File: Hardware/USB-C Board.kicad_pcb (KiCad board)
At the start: 2 copper layers, 34 x 34 mm, 52 parts, among them J1 USB_C_Receptacle_USB2.0, J2 Conn_01x04_Male, J3 Conn_01x02_Male, J4 Conn_01x02_Male, J5 Conn_01x02_Male, J6 Conn_01x02_Male, J9 Conn_01x04_MountingPin, Q1 DMP3013SFV, SW1 SW_Push, U1 AMS1117-3.3, U3 STUSB4500QTR

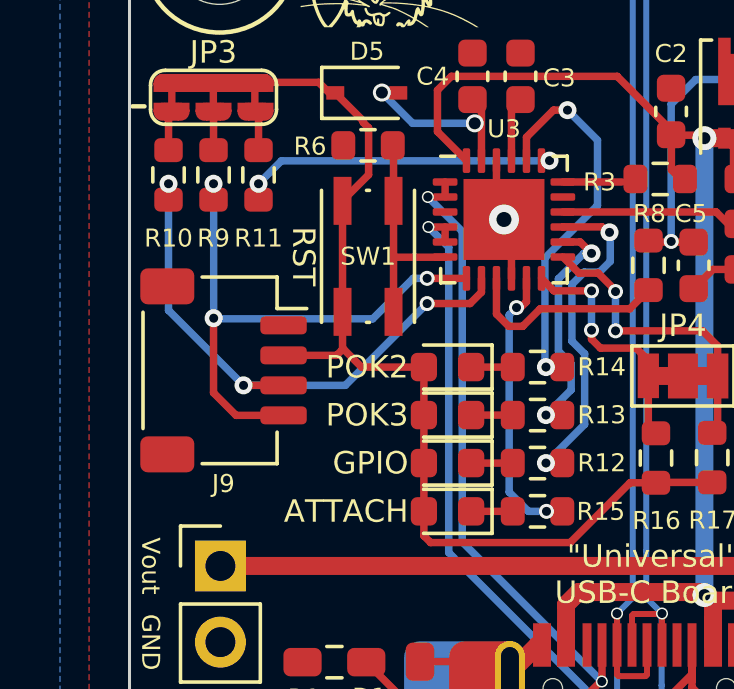
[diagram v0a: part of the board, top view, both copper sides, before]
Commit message: starting on controller boards
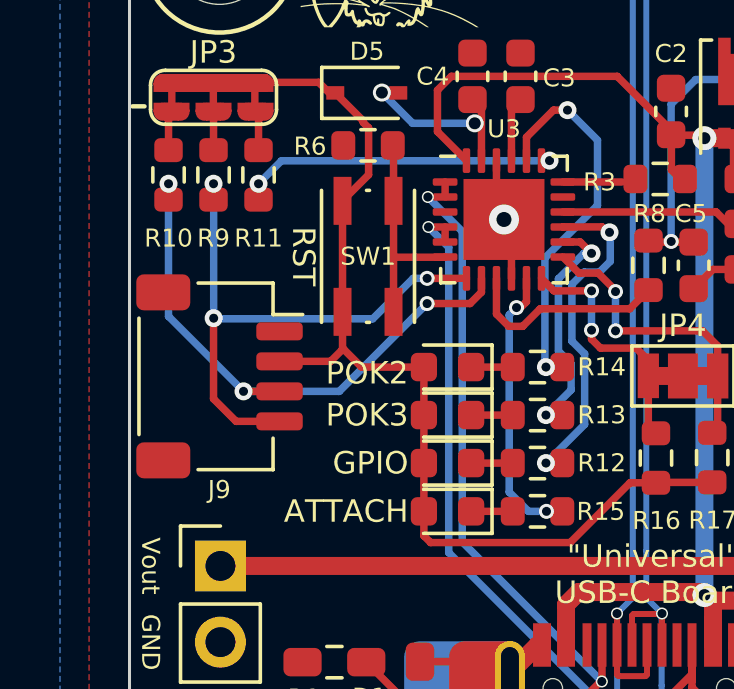
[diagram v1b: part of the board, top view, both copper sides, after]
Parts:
- moved J9 0.24 mm to (86.0, 87.0)
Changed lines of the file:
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@@
   )
   (footprint "Tinker:JST_SH_SM04B-SRSS-TB_1x04-1MP_P1.00mm_Horizontal" (layer "F.Cu")
-    (at 86.13441 86.8 -90)
+    (at 86 87 -90)
     (descr "JST SH series connector, SM04B-SRSS-TB (http://www.jst-mfg.com/product/pdf/eng/eSH.pdf), generated with kicad-footprint-generator")
     (tags "connector JST SH top entry")
@@
       (effects (font (size 0.6 0.6) (thickness 0.15)))
     )
-    (fp_text value "Conn_01x04_MountingPin" (at 0 3.98 -90) (layer "F.Fab") hide
+    (fp_text value "Conn_01x04_MountingPin" (at 0 3.98 90) (layer "F.Fab") hide
       (effects (font (size 1 1) (thickness 0.15)))
     )
-    (fp_text user "${REFERENCE}" (at 0 0 -90) (layer "F.Fab") hide
+    (fp_text user "${REFERENCE}" (at 0 0 90) (layer "F.Fab") hide
       (effects (font (size 1 1) (thickness 0.15)))
     )
@@
     (effects (font (size 0.6 0.6) (thickness 0.125)))
   )
-  (gr_text "POK2" (at 92.298126 86.690928) (layer "F.SilkS")
+  (gr_text "POK2" (at 92.298126 86.890928) (layer "F.SilkS")
     (effects (font (size 0.75 0.75) (thickness 0.15)) (justify right))
   )
@@
   (segment (start 99.675221 84.748251) (end 100.29898 84.124492) (width 0.25) (layer "F.Cu") (net 16))
   (segment (start 96.105782 85.332753) (end 96.690284 84.748251) (width 0.25) (layer "F.Cu") (net 16))
-  (segment (start 85.8 87.548526) (end 85.8 85.067178) (width 0.25) (layer "F.Cu") (net 17))
-  (segment (start 86.551474 88.3) (end 88.13441 88.3) (width 0.25) (layer "F.Cu") (net 17))
+  (segment (start 85.8 87.748526) (end 85.8 85.267178) (width 0.25) (layer "F.Cu") (net 17))
+  (segment (start 86.551474 88.5) (end 88.13441 88.5) (width 0.25) (layer "F.Cu") (net 17))
   (segment (start 85.8 85.067178) (end 85.805394 85.061784) (width 0.25) (layer "F.Cu") (net 17))
-  (segment (start 85.8 87.548526) (end 86.551474 88.3) (width 0.25) (layer "F.Cu") (net 17))
+  (segment (start 85.8 87.748526) (end 86.551474 88.5) (width 0.25) (layer "F.Cu") (net 17))
   (segment (start 94.231969 83.73369) (end 92.819469 83.73369) (width 0.25) (layer "F.Cu") (net 17))
   (via (at 92.919469 83.73369) (size 0.5) (drill 0.3) (layers "F.Cu" "B.Cu") (net 17))
@@
   (segment (start 85.805394 80.585394) (end 85.8 80.58) (width 0.25) (layer "B.Cu") (net 17))
   (segment (start 94.731969 83.73369) (end 94.731969 84.194198) (width 0.25) (layer "F.Cu") (net 18))
-  (segment (start 86.8 87.3) (end 88.13441 87.3) (width 0.25) (layer "F.Cu") (net 18))
+  (segment (start 86.8 87.5) (end 88.13441 87.5) (width 0.25) (layer "F.Cu") (net 18))
   (segment (start 94.731969 84.194198) (end 94.352345 84.573822) (width 0.25) (layer "F.Cu") (net 18))
   (segment (start 94.352345 84.573822) (end 92.819469 84.573822) (width 0.25) (layer "F.Cu") (net 18))
   (via (at 84.3 80.58) (size 0.6) (drill 0.3) (layers "F.Cu" "B.Cu") (net 18))
   (via (at 92.919469 84.573822) (size 0.5) (drill 0.3) (layers "F.Cu" "B.Cu") (net 18))
-  (via (at 86.8 87.3) (size 0.6) (drill 0.3) (layers "F.Cu" "B.Cu") (net 18))
-  (segment (start 90.193291 87.3) (end 92.919469 84.573822) (width 0.25) (layer "B.Cu") (net 18))
-  (segment (start 84.3 84.8) (end 84.3 80.58) (width 0.25) (layer "B.Cu") (net 18))
-  (segment (start 86.8 87.3) (end 90.193291 87.3) (width 0.25) (layer "B.Cu") (net 18))
-  (segment (start 86.8 87.3) (end 84.3 84.8) (width 0.25) (layer "B.Cu") (net 18))
+  (via (at 86.8 87.5) (size 0.6) (drill 0.3) (layers "F.Cu" "B.Cu") (net 18))
+  (segment (start 86.801247 87.501247) (end 89.992045 87.501247) (width 0.25) (layer "B.Cu") (net 18))
+  (segment (start 84.3 85) (end 84.3 80.58) (width 0.25) (layer "B.Cu") (net 18))
+  (segment (start 86.8 87.5) (end 86.801247 87.501247) (width 0.25) (layer "B.Cu") (net 18))
+  (segment (start 89.992045 87.501247) (end 92.919469 84.573822) (width 0.25) (layer "B.Cu") (net 18))
+  (segment (start 86.8 87.5) (end 84.3 85) (width 0.25) (layer "B.Cu") (net 18))
   (segment (start 98.749917 82.018851) (end 99.008319 82.277253) (width 0.25) (layer "F.Cu") (net 19))
   (segment (start 97.446808 82.018851) (end 98.749917 82.018851) (width 0.25) (layer "F.Cu") (net 19))
@@
   (segment (start 100.561666 90.534091) (end 100.548181 90.547576) (width 0.25) (layer "F.Cu") (net 21))
   (segment (start 90.734379 86.690928) (end 90.145703 86.102252) (width 0.25) (layer "F.Cu") (net 21))
+  (segment (start 89.702252 86.5) (end 90.1 86.102252) (width 0.25) (layer "F.Cu") (net 21))
+  (segment (start 88.13441 86.5) (end 89.702252 86.5) (width 0.25) (layer "F.Cu") (net 21))
   (segment (start 90.1 86.102252) (end 90.1 84.85) (width 0.25) (layer "F.Cu") (net 21))
   (segment (start 92.8125 86.690928) (end 90.734379 86.690928) (width 0.25) (layer "F.Cu") (net 21))
@@
   (segment (start 89.306161 77.19985) (end 89.657663 77.551352) (width 0.25) (layer "F.Cu") (net 21))
   (segment (start 99.682726 90.547576) (end 97.689391 92.540911) (width 0.25) (layer "F.Cu") (net 21))
-  (segment (start 88.13441 86.3) (end 89.902252 86.3) (width 0.25) (layer "F.Cu") (net 21))
   (segment (start 90.96983 78.717587) (end 90.96983 80.28017) (width 0.25) (layer "F.Cu") (net 21))
   (segment (start 90.1 86.102252) (end 90.145703 86.102252) (width 0.25) (layer "F.Cu") (net 21))
@@
   (segment (start 102.422576 90.534091) (end 100.561666 90.534091) (width 0.25) (layer "F.Cu") (net 21))
   (segment (start 92.8125 92.316297) (end 93.037114 92.540911) (width 0.25) (layer "F.Cu") (net 21))
-  (segment (start 89.902252 86.3) (end 90.1 86.102252) (width 0.25) (layer "F.Cu") (net 21))
   (segment (start 97.689391 92.540911) (end 93.037114 92.540911) (width 0.25) (layer "F.Cu") (net 21))
   (segment (start 90.96983 80.28017) (end 90.1 81.15) (width 0.25) (layer "F.Cu") (net 21))

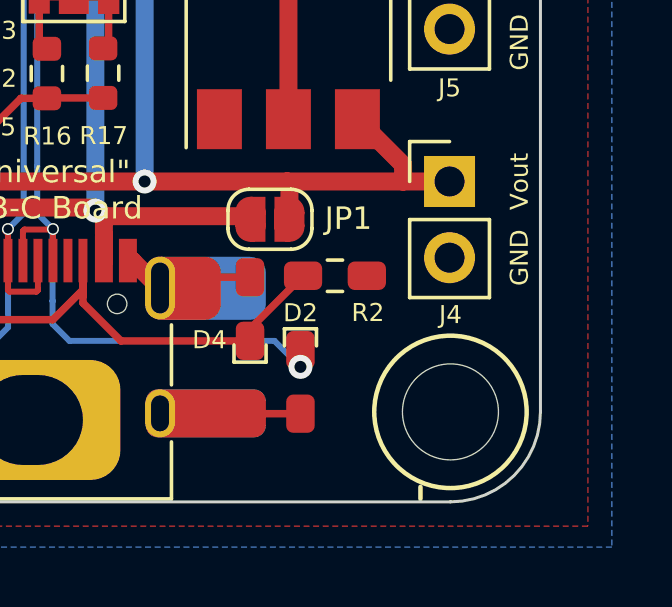
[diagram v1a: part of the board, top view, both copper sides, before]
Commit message: ...
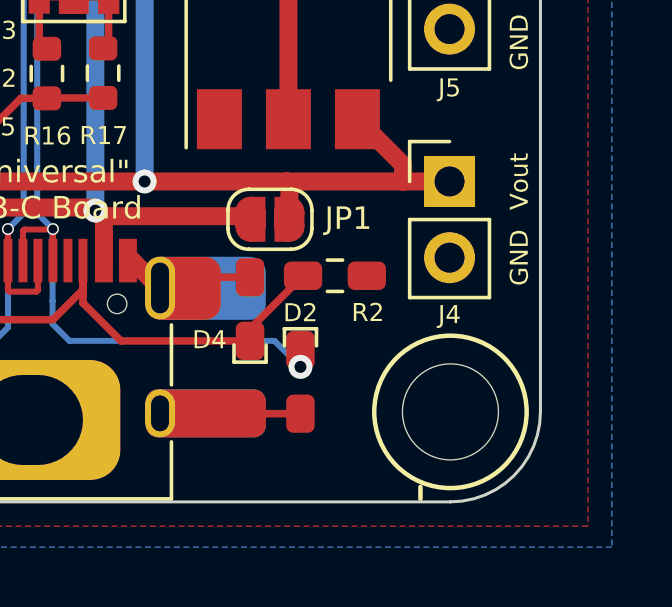
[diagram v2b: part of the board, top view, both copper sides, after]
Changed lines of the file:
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@@
-    )
-  )
-  (footprint "Tinker:PinHeader_1x02_P2.54mm_Vertical" (layer "F.Cu")
-    (at 113.97 93.32)
-    (descr "Through hole straight pin header, 1x02, 2.54mm pitch, single row")
-    (tags "Through hole pin header THT 1x02 2.54mm single row")
-    (property "Sheetfile" "USB-C Board.kicad_sch")
-    (property "Sheetname" "")
-    (attr through_hole)
-    (fp_text reference "J4" (at 0.03 4.44169) (layer "F.SilkS")
-      (effects (font (size 0.6 0.6) (thickness 0.15)))
-    )
-    (fp_text value "Conn_01x02_Male" (at 0 4.87) (layer "F.Fab") hide
-      (effects (font (size 1 1) (thickness 0.15)))
-    )
-    (fp_text user "${REFERENCE}" (at 0 1.27 90) (layer "F.Fab")
-      (effects (font (size 1 1) (thickness 0.15)))
-    )
-    (fp_line (start -1.33 1.27) (end -1.33 3.87) (layer "F.SilkS") (width 0.12))
-    (fp_line (start -1.33 -1.33) (end 0 -1.33) (layer "F.SilkS") (width 0.12))
-    (fp_line (start -1.33 0) (end -1.33 -1.33) (layer "F.SilkS") (width 0.12))
-    (fp_line (start -1.33 1.27) (end 1.33 1.27) (layer "F.SilkS") (width 0.12))
-    (fp_line (start 1.33 1.27) (end 1.33 3.87) (layer "F.SilkS") (width 0.12))
-    (fp_line (start -1.33 3.87) (end 1.33 3.87) (layer "F.SilkS") (width 0.12))
-    (fp_line (start -1.4 -1.4) (end -1.4 3.95) (layer "F.CrtYd") (width 0.05))
-    (fp_line (start 1.4 3.95) (end 1.4 -1.4) (layer "F.CrtYd") (width 0.05))
-    (fp_line (start -1.4 3.95) (end 1.4 3.95) (layer "F.CrtYd") (width 0.05))
-    (fp_line (start 1.4 -1.4) (end -1.4 -1.4) (layer "F.CrtYd") (width 0.05))
-    (fp_line (start 1.27 3.81) (end -1.27 3.81) (layer "F.Fab") (width 0.1))
-    (fp_line (start 1.27 -1.27) (end 1.27 3.81) (layer "F.Fab") (width 0.1))
-    (fp_line (start -1.27 3.81) (end -1.27 -0.635) (layer "F.Fab") (width 0.1))
-    (fp_line (start -0.635 -1.27) (end 1.27 -1.27) (layer "F.Fab") (width 0.1))
-    (fp_line (start -1.27 -0.635) (end -0.635 -1.27) (layer "F.Fab") (width 0.1))
-    (pad "1" thru_hole rect (at 0 0) (size 1.7 1.7) (drill 1) (layers *.Cu *.Mask)
-      (net 26 "Vout") (pinfunction "Pin_1") (pintype "passive"))
-    (pad "2" thru_hole oval (at 0 2.54) (size 1.7 1.7) (drill 1) (layers *.Cu *.Mask)
-      (net 24 "GND") (pinfunction "Pin_2") (pintype "passive"))
-    (model "${KICAD6_3DMODEL_DIR}/Connector_PinHeader_2.54mm.3dshapes/PinHeader_1x02_P2.54mm_Vertical.wrl"
-      (offset (xyz 0 0 0))
-      (scale (xyz 1 1 1))
-      (rotate (xyz 0 0 0))
     )
   )
@@
     )
   )
+  (footprint "Tinker:PinHeader_1x02_P2.54mm_Vertical" (layer "F.Cu")
+    (at 113.97 93.32)
+    (descr "Through hole straight pin header, 1x02, 2.54mm pitch, single row")
+    (tags "Through hole pin header THT 1x02 2.54mm single row")
+    (property "Sheetfile" "USB-C Board.kicad_sch")
+    (property "Sheetname" "")
+    (attr through_hole)
+    (fp_text reference "J4" (at 0 4.44169) (layer "F.SilkS")
+      (effects (font (size 0.6 0.6) (thickness 0.15)))
+    )
+    (fp_text value "Conn_01x02_Male" (at 0 4.87) (layer "F.Fab") hide
+      (effects (font (size 1 1) (thickness 0.15)))
+    )
+    (fp_text user "${REFERENCE}" (at 0 1.27 90) (layer "F.Fab")
+      (effects (font (size 1 1) (thickness 0.15)))
+    )
+    (fp_line (start -1.33 3.87) (end 1.33 3.87) (layer "F.SilkS") (width 0.12))
+    (fp_line (start 1.33 1.27) (end 1.33 3.87) (layer "F.SilkS") (width 0.12))
+    (fp_line (start -1.33 0) (end -1.33 -1.33) (layer "F.SilkS") (width 0.12))
+    (fp_line (start -1.33 1.27) (end -1.33 3.87) (layer "F.SilkS") (width 0.12))
+    (fp_line (start -1.33 -1.33) (end 0 -1.33) (layer "F.SilkS") (width 0.12))
+    (fp_line (start -1.33 1.27) (end 1.33 1.27) (layer "F.SilkS") (width 0.12))
+    (fp_line (start 1.4 -1.4) (end -1.4 -1.4) (layer "F.CrtYd") (width 0.05))
+    (fp_line (start -1.4 -1.4) (end -1.4 3.95) (layer "F.CrtYd") (width 0.05))
+    (fp_line (start 1.4 3.95) (end 1.4 -1.4) (layer "F.CrtYd") (width 0.05))
+    (fp_line (start -1.4 3.95) (end 1.4 3.95) (layer "F.CrtYd") (width 0.05))
+    (fp_line (start 1.27 -1.27) (end 1.27 3.81) (layer "F.Fab") (width 0.1))
+    (fp_line (start -1.27 3.81) (end -1.27 -0.635) (layer "F.Fab") (width 0.1))
+    (fp_line (start 1.27 3.81) (end -1.27 3.81) (layer "F.Fab") (width 0.1))
+    (fp_line (start -1.27 -0.635) (end -0.635 -1.27) (layer "F.Fab") (width 0.1))
+    (fp_line (start -0.635 -1.27) (end 1.27 -1.27) (layer "F.Fab") (width 0.1))
+    (pad "1" thru_hole rect (at 0 0) (size 1.7 1.7) (drill 1) (layers *.Cu *.Mask)
+      (net 26 "Vout") (pinfunction "Pin_1") (pintype "passive"))
+    (pad "2" thru_hole oval (at 0 2.54) (size 1.7 1.7) (drill 1) (layers *.Cu *.Mask)
+      (net 24 "GND") (pinfunction "Pin_2") (pintype "passive"))
+    (model "${KICAD6_3DMODEL_DIR}/Connector_PinHeader_2.54mm.3dshapes/PinHeader_1x02_P2.54mm_Vertical.wrl"
+      (offset (xyz 0 0 0))
+      (scale (xyz 1 1 1))
+      (rotate (xyz 0 0 0))
+    )
+  )
